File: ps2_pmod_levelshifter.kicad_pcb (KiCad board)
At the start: 2 copper layers, 35.5 x 23 mm, 4 parts, among them J1 PS/2, J2 PMOD, J3 EXT_POWER

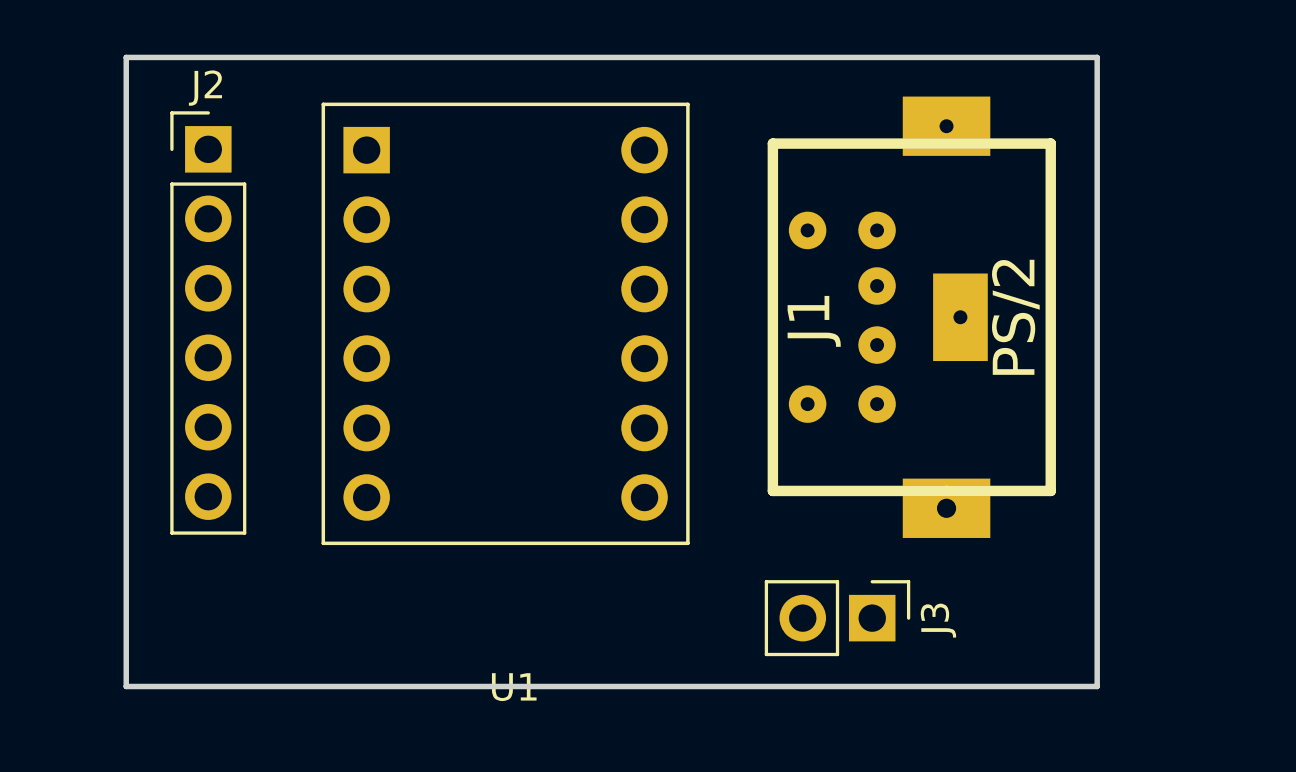
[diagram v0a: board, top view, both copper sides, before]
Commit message: update design
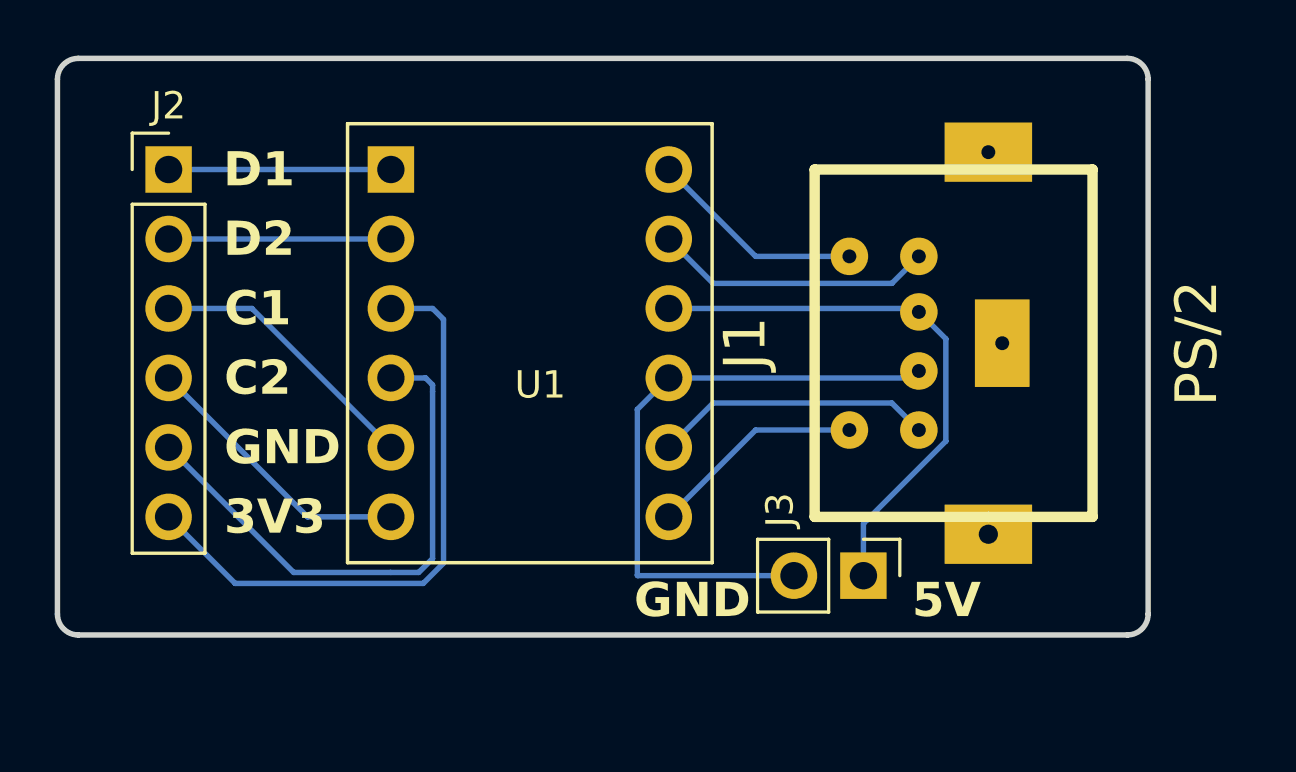
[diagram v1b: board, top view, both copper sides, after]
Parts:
- moved J1 1.80 mm to (158.8, 91.9)
- moved J2 1.63 mm to (130.0, 85.6)
- moved J3 1.59 mm to (155.5, 100.4)
- moved U1 1.13 mm to (143.6, 91.9)
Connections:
- J1 pad 3: /PS/2_CLK -> VCC_5V
- J1 pad 4: /PS/2_CLK- -> GND_5V
- J1 pad 5: VCC_5V -> /PS/2_CLK
- J1 pad 6: GND_5V -> /PS/2_CLK-
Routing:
- net GND_5V: track 0.00 -> 22.7 mm
- net VCC_3V3: track 0.00 -> 22.4 mm
- net VCC_5V: track 0.00 -> 20.5 mm
- net /PMOD_CLK-: track 0.00 -> 10.2 mm
- net /PMOD_CLK: track 0.00 -> 10.2 mm
- net /PS/2_DATA-: track 0.00 -> 10.2 mm
- net /PS/2_CLK: track 0.00 -> 10.2 mm
- net GND_3V3: track 0.00 -> 10.0 mm
- net /PS/2_DATA: track 0.00 -> 7.92 mm
- net /PS/2_CLK-: track 0.00 -> 7.92 mm
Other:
- board size 35.5 x 23 mm -> 39.9 x 21.1 mm
- board text added: "3V3"
- board text added: "5V"
- board text added: "C1"
- board text added: "C2"
- board text added: "D1"
- board text added: "D2"
- board text added: "GND"
